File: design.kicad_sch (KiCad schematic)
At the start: 19 parts, among them J1 Conn_02x02_Counter_Clockwise, J2 Conn_02x02_Counter_Clockwise, J3 Conn_02x02_Counter_Clockwise, U1 TPS63900

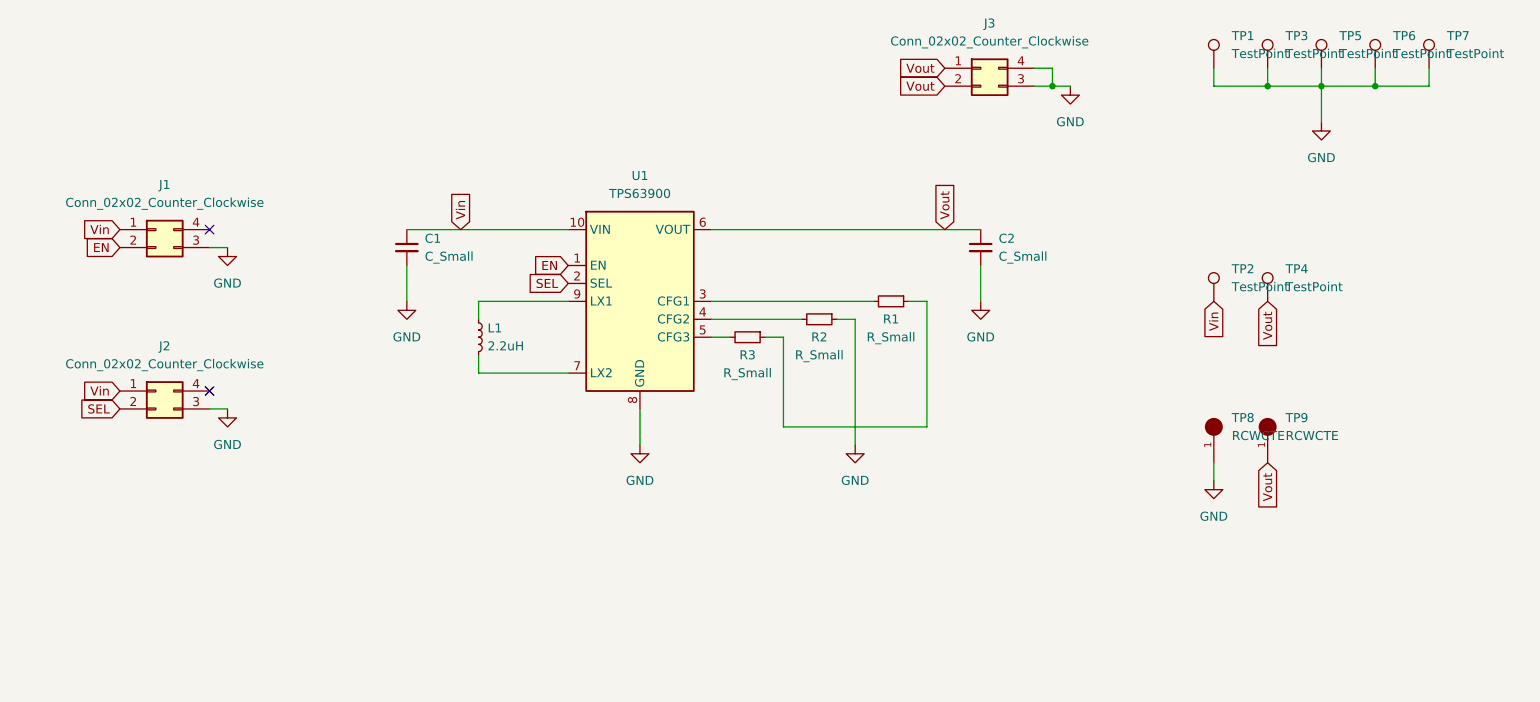
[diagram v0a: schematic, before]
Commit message: update
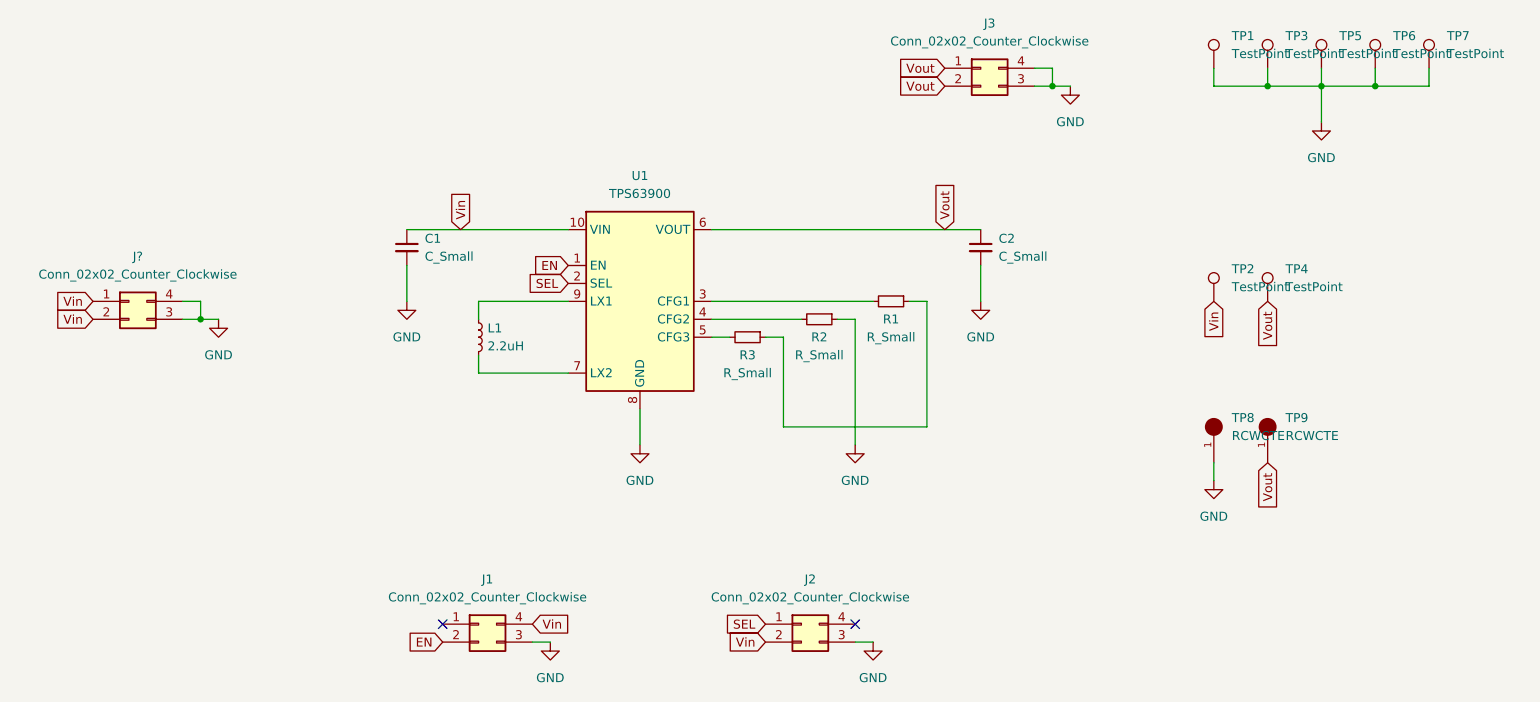
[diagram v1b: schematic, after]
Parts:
- added J?: Conn_02x02_Counter_Clockwise, Connector_PinSocket_2.54mm:PinSocket_2x02_P2.54mm_Vertical, symbol Connector_Generic:Conn_02x02_Counter_Clockwise
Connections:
- net GND: now also J?.3 (Pin_3), J?.4 (Pin_4)
- net SEL: now also J2.1 (Pin_1); no longer J2.2 (Pin_2)
- net Vin: now also J1.4 (Pin_4), J2.2 (Pin_2), J?.1 (Pin_1), J?.2 (Pin_2); no longer J1.1 (Pin_1), J2.1 (Pin_1)
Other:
- moved on the sheet: J1, J2
